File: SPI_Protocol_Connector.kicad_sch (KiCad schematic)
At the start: 7 parts, among them J13 Conn_01x03_Pin, U10 TXB0104PW, U9 TXB0104PW

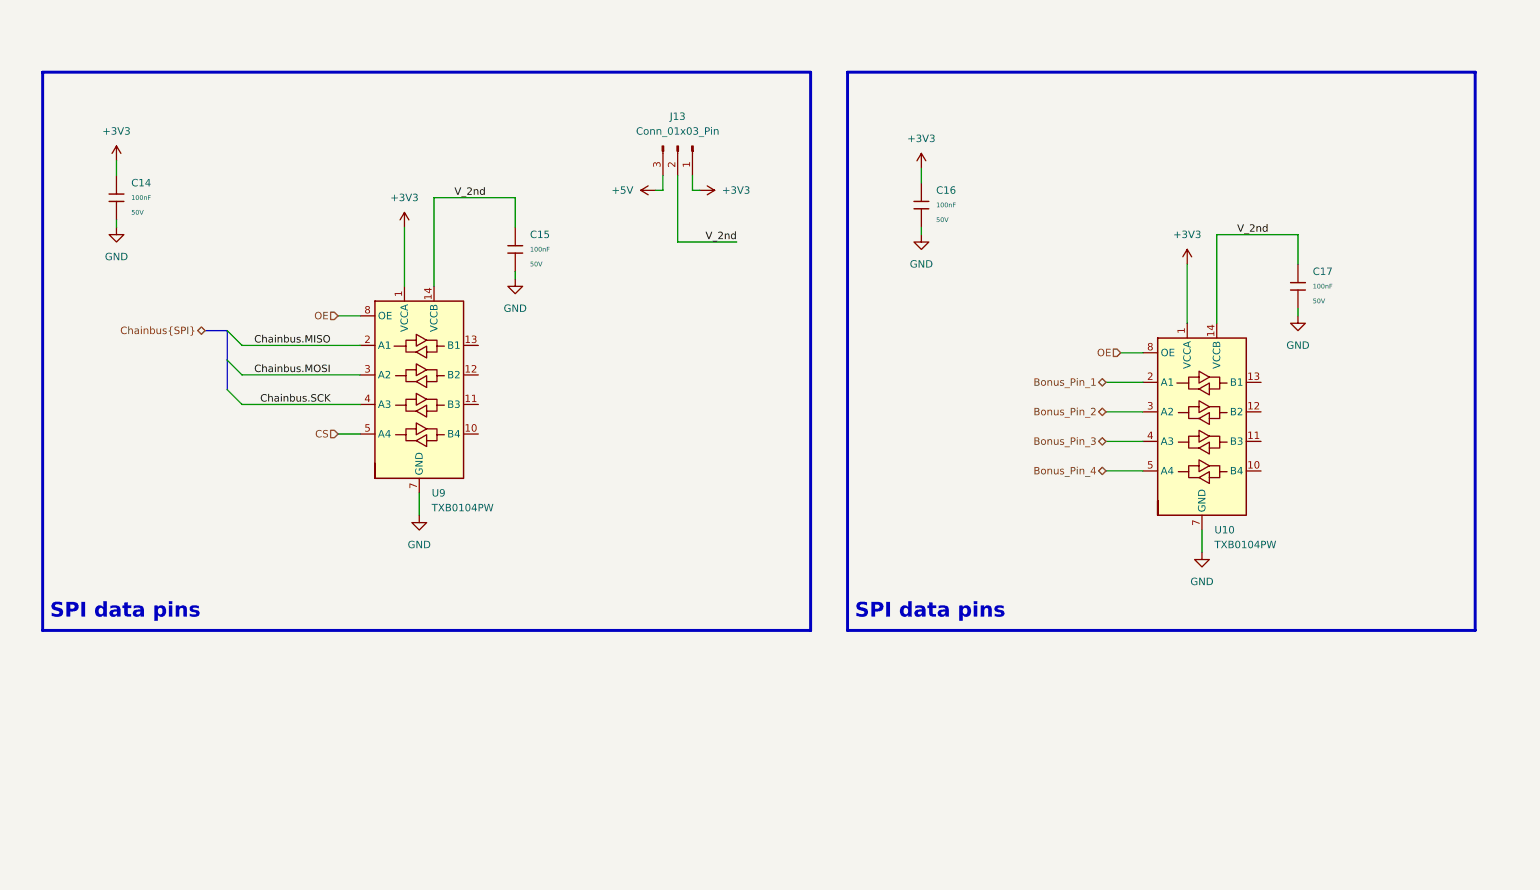
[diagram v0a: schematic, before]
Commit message: schematic done
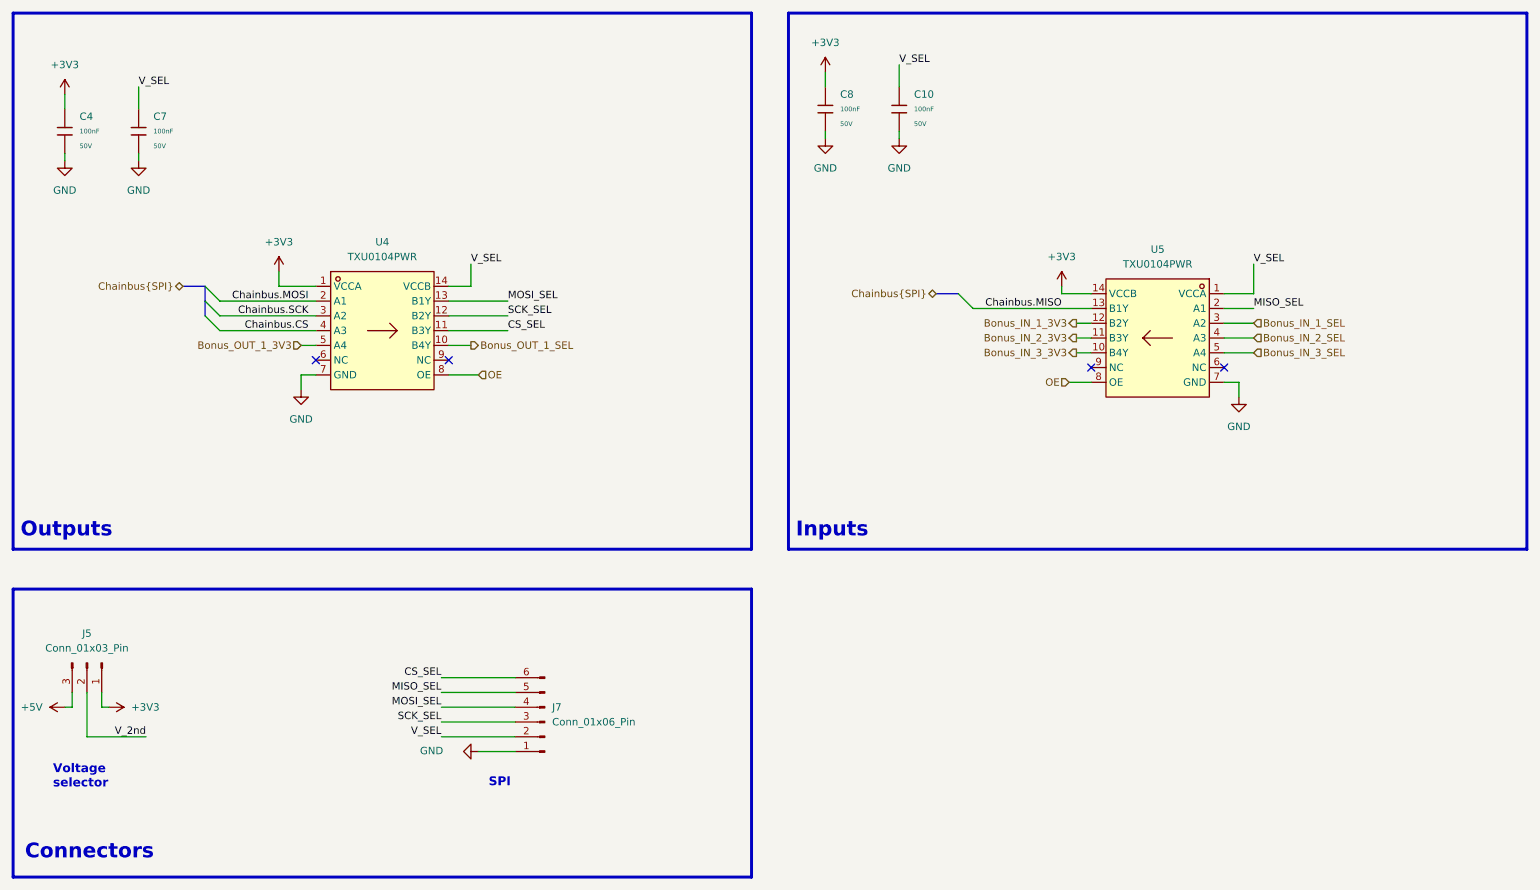
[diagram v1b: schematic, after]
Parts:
- removed C14, C15, C16, C17: 100nF, PCM_JLCPCB:C_0603, symbol PCM_JLCPCB-Capacitors:0603,100nF
- removed J13: Conn_01x03_Pin, Connector_PinSocket_2.54mm:PinSocket_1x03_P2.54mm_Vertical, symbol Connector:Conn_01x03_Pin
- removed U10, U9: TXB0104PW, Package_SO:TSSOP-14_4.4x5mm_P0.65mm, symbol Logic_LevelTranslator:TXB0104PW
- added C10, C4, C7, C8: 100nF, PCM_JLCPCB:C_0603, symbol PCM_JLCPCB-Capacitors:0603,100nF
- added J5: Conn_01x03_Pin, Connector_PinSocket_2.54mm:PinSocket_1x03_P2.54mm_Vertical, symbol Connector:Conn_01x03_Pin
- added J7: Conn_01x06_Pin, Connector_JST:JST_XH_S6B-XH-A_1x06_P2.50mm_Horizontal, symbol Connector:Conn_01x06_Pin
- added U4, U5: TXU0104PWR, TXU0104PWR:TSSOP-14_L5.0-W4.4-P0.65-LS6.4-BL, symbol TXU0104PWR:TXU0104PWR
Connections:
- net +3V3: now also C4.1, C8.1, J5.1 (Pin_1), U4.1 (VCCA), U5.14 (VCCB)
- net +5V: now also J5.3 (Pin_3)
- net Chainbus.MISO: now also U5.13 (B1Y)
- net Chainbus.MOSI: now also U4.2 (A1)
- net Chainbus.SCK: now also U4.3 (A2)
- net GND: now also C10.2, C4.2, C7.2, C8.2, J7.1 (Pin_1), U4.7 (GND), U5.7 (GND)
- net OE: now also U4.8 (OE), U5.8 (OE)
- net V_2nd: now also J5.2 (Pin_2)
- new net Bonus_IN_1_3V3: U5.12 (B2Y)
- new net Bonus_IN_1_SEL: U5.3 (A2)
- new net Bonus_IN_2_3V3: U5.11 (B3Y)
- new net Bonus_IN_2_SEL: U5.4 (A3)
- new net Bonus_IN_3_3V3: U5.10 (B4Y)
- new net Bonus_IN_3_SEL: U5.5 (A4)
- new net Bonus_OUT_1_3V3: U4.5 (A4)
- new net Bonus_OUT_1_SEL: U4.10 (B4Y)
- new net CS_SEL: J7.6 (Pin_6), U4.11 (B3Y)
- new net Chainbus.CS: U4.4 (A3)
- new net MISO_SEL: J7.5 (Pin_5), U5.2 (A1)
- new net MOSI_SEL: J7.4 (Pin_4), U4.13 (B1Y)
- new net SCK_SEL: J7.3 (Pin_3), U4.12 (B2Y)
- new net V_SEL: C10.1, C7.1, J7.2 (Pin_2), U4.14 (VCCB), U5.1 (VCCA)
- no-connect marks 0 -> 4
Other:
- note added: "Connectors"
- note added: "Inputs"
- note added: "Outputs"
- note added: "SPI"
- note added: "Voltage selector"
- note removed: "SPI data pins"
- title: MMS3 Hat template small (Change Me) -> MMS3 hat protocol
